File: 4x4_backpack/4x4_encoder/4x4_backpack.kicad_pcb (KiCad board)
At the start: 2 copper layers, 76.2 x 76.2 mm, 38 parts, among them J1 Conn_01x04, J11 Conn_01x01, J12 Conn_01x01, J13 Conn_01x01, J14 Conn_01x01, J15 Conn_01x01, J16 Conn_01x01, J2 Conn_01x04, J3 Conn_01x04, J4 Conn_01x04, J5 Conn_01x04, J6 Conn_01x04, J7 Conn_01x04, J8 Conn_01x04, SW1 Rotary_Encoder_Switch, SW2 Rotary_Encoder_Switch, SW3 Rotary_Encoder_Switch, SW4 Rotary_Encoder_Switch

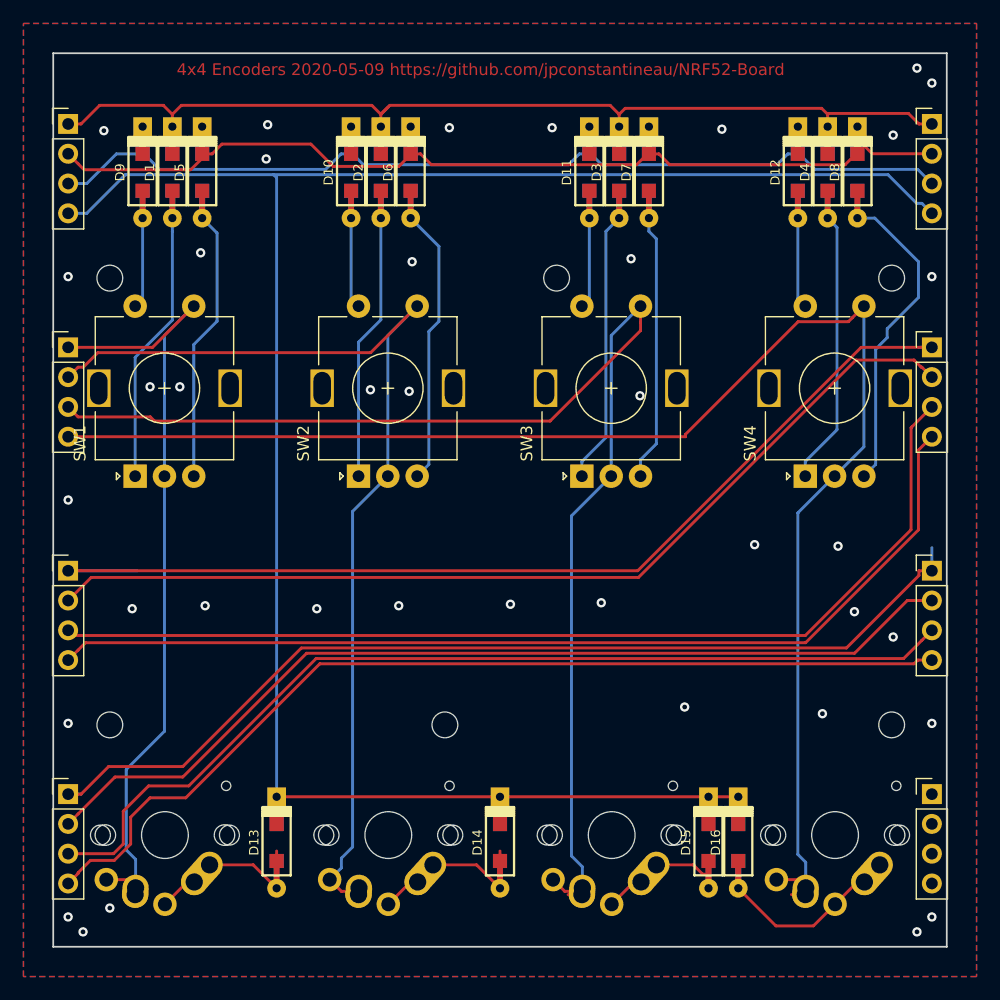
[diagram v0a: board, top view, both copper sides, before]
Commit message: added BlueHand to docs
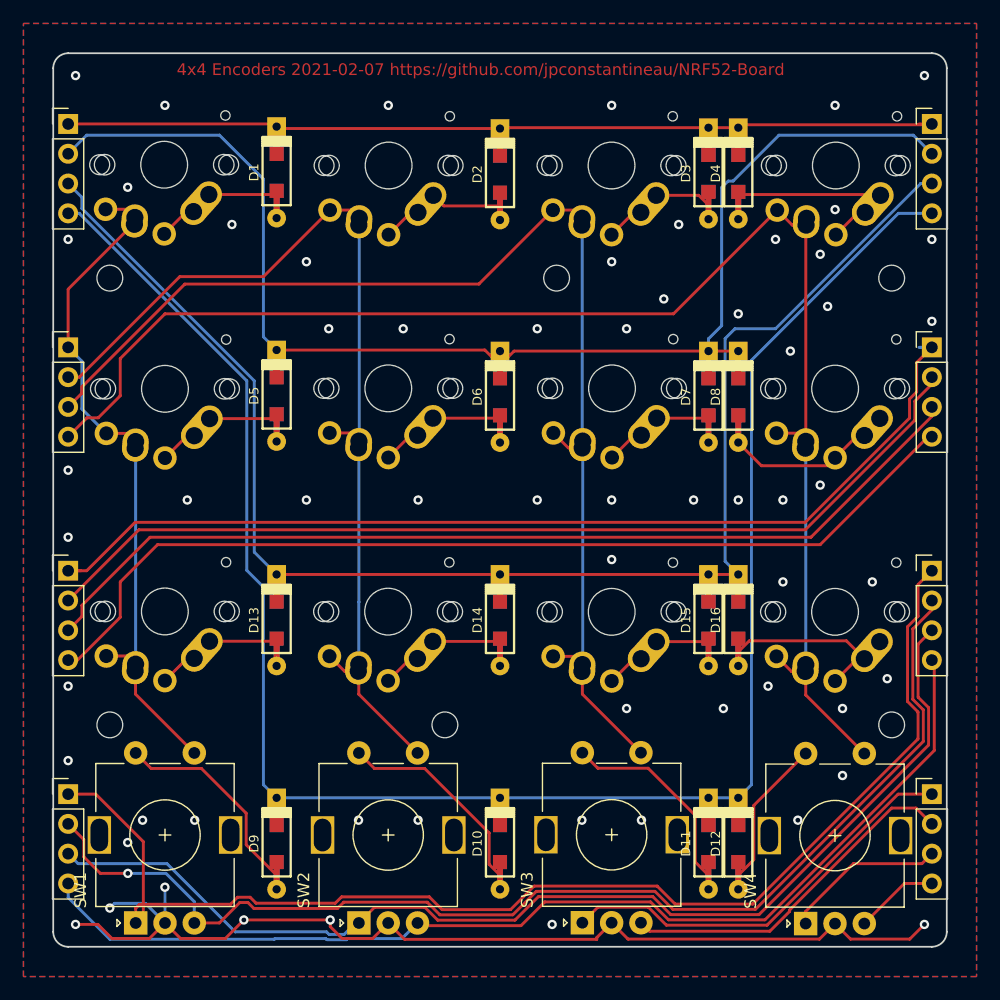
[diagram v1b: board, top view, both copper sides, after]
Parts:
- added S1: CHERRY_MX, footprints:MX-Alps-Choc-1U, F.Cu at (85.7, 85.7)
- added S2: CHERRY_MX, footprints:MX-Alps-Choc-1U, F.Cu at (85.7, 104.8)
- added S3: CHERRY_MX, footprints:MX-Alps-Choc-1U, F.Cu at (104.8, 85.8)
- added S4: CHERRY_MX, footprints:MX-Alps-Choc-1U, F.Cu at (104.8, 104.8)
- added S5: CHERRY_MX, footprints:MX-Alps-Choc-1U, F.Cu at (123.8, 85.8)
- added S6: CHERRY_MX, footprints:MX-Alps-Choc-1U, F.Cu at (123.9, 104.8)
- added S7: CHERRY_MX, footprints:MX-Alps-Choc-1U, F.Cu at (142.9, 85.8)
- added S8: CHERRY_MX, footprints:MX-Alps-Choc-1U, F.Cu at (142.9, 104.8)
- moved D10 58.6 mm to (114.3, 143.6)
- moved D9 58.4 mm to (95.2, 143.6)
- moved D11 58.1 mm to (132.1, 143.6)
- moved D12 57.5 mm to (134.6, 143.6)
- moved SW4 38.2 mm to (140.4, 150.4)
- moved SW1 38.1 mm to (83.2, 150.4)
- moved SW2 38.1 mm to (102.3, 150.4)
- moved SW3 38.1 mm to (121.3, 150.4)
- moved D8 21.7 mm to (134.6, 105.5)
- moved D6 20.6 mm to (114.3, 105.5)
- moved D5 20.1 mm to (95.2, 105.4)
- moved D7 19.8 mm to (132.1, 105.5)
- moved S13 19.1 mm to (85.7, 123.8)
- moved S14 19.1 mm to (104.8, 123.8)
- moved S15 19.0 mm to (123.8, 123.8)
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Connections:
- D10 pad 1: ROW3 -> ROW4
- D11 pad 1: ROW3 -> ROW4
- D12 pad 1: ROW3 -> ROW4
- D13 pad 1: ROW4 -> ROW3
- D14 pad 1: ROW4 -> ROW3
- D15 pad 1: ROW4 -> ROW3
- D16 pad 1: ROW4 -> ROW3
- D9 pad 1: ROW3 -> ROW4
- J8 pad 1: (no net) -> COL13
- J8 pad 2: (no net) -> COL14
- J8 pad 3: (no net) -> COL15
- J8 pad 4: (no net) -> COL16
- SW1 pad A: Net-(D1-Pad2) -> COL9
- SW1 pad B: Net-(D5-Pad2) -> COL10
- SW1 pad C: COL1 -> GND
- SW2 pad A: Net-(D2-Pad2) -> COL11
- SW2 pad B: Net-(D6-Pad2) -> COL12
- SW2 pad C: COL2 -> GND
- SW3 pad A: Net-(D3-Pad2) -> COL13
- SW3 pad B: Net-(D7-Pad2) -> COL14
- SW3 pad C: COL3 -> GND
- SW4 pad A: Net-(D4-Pad2) -> COL15
- SW4 pad B: Net-(D8-Pad2) -> COL16
- SW4 pad C: COL4 -> GND
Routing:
- net GND: track 0.00 -> 88.2 mm, vias 39 -> 62
- net ROW3: track 82.6 -> 125.2 mm
- net COL13: track 0.00 -> 35.6 mm
- net COL14: track 0.00 -> 30.1 mm
- net ROW2: track 84.1 -> 109.2 mm
- net COL9: track 84.9 -> 107.4 mm
- net COL10: track 81.6 -> 100.4 mm, vias 0 -> 1
- net ROW4: track 170.4 -> 155.5 mm
- net COL15: track 0.00 -> 13.8 mm
- net Net-(D3-Pad2): track 23.3 -> 10.0 mm
- net Net-(D7-Pad2): track 22.8 -> 9.72 mm
- net Net-(D6-Pad2): track 23.8 -> 11.0 mm
- net Net-(D8-Pad2): track 27.7 -> 14.9 mm
- net COL11: track 83.2 -> 95.7 mm
- net Net-(D5-Pad2): track 23.4 -> 11.1 mm
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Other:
- outline, holes or cut-outs redrawn
- board text added: "4x4 Encoders 2021-02-07 https://github.com/jpconstantineau/NRF52-Board"
- board text added: "Encoders"
- board text added: "Encoders need Standoffs for GND Connection."
- board text removed: "4x4 Encoders 2020-05-09 https://github.com/jpconstantineau/NRF52-Board"
- board text removed: "Cols after"
- board text removed: "Cols last"
